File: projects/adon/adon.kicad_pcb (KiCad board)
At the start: 2 copper layers, 55.9 x 30.5 mm, 31 parts, among them IC1 STM32F030F4, P1 BATTERY, P2 SWD, Q1 2N3704, SW1 POWER, SW2 BUTTON0, SW3 BUTTON1, SW4 BUTTON2, SW5 BUTTON3

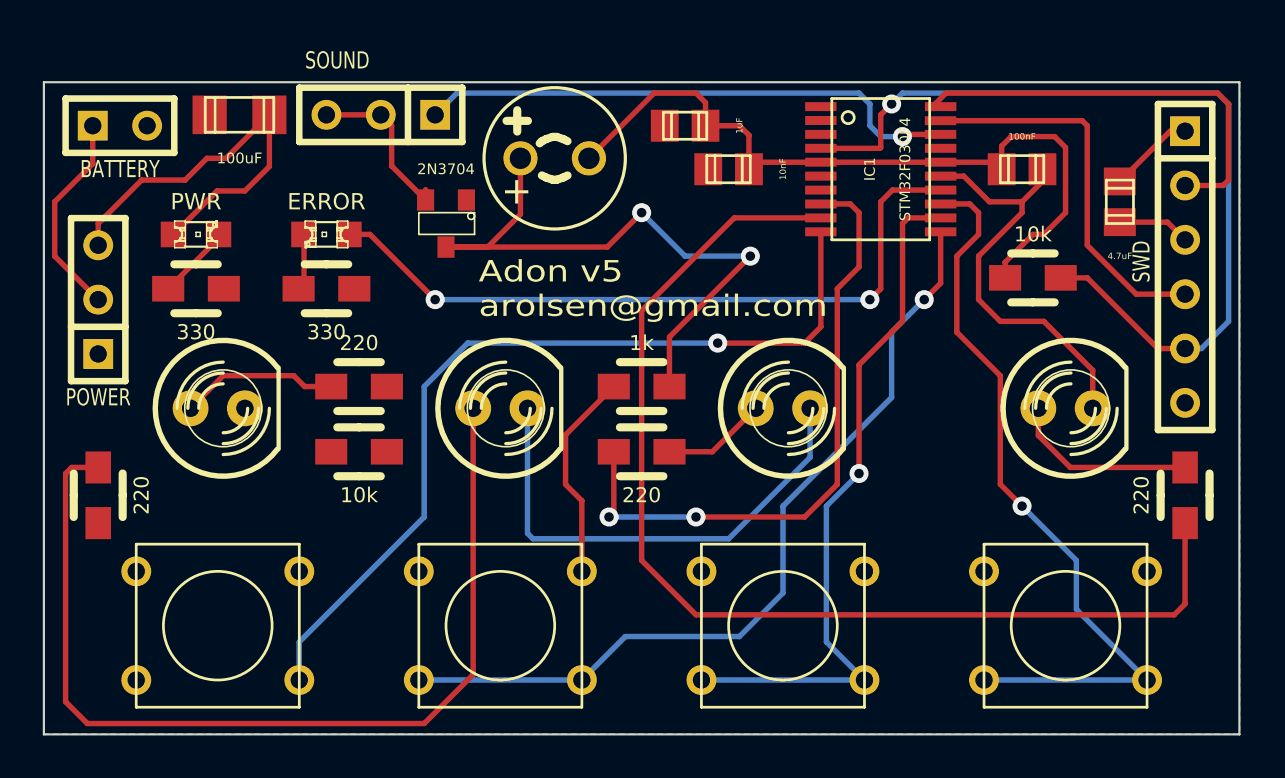
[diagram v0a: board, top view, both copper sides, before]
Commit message: done
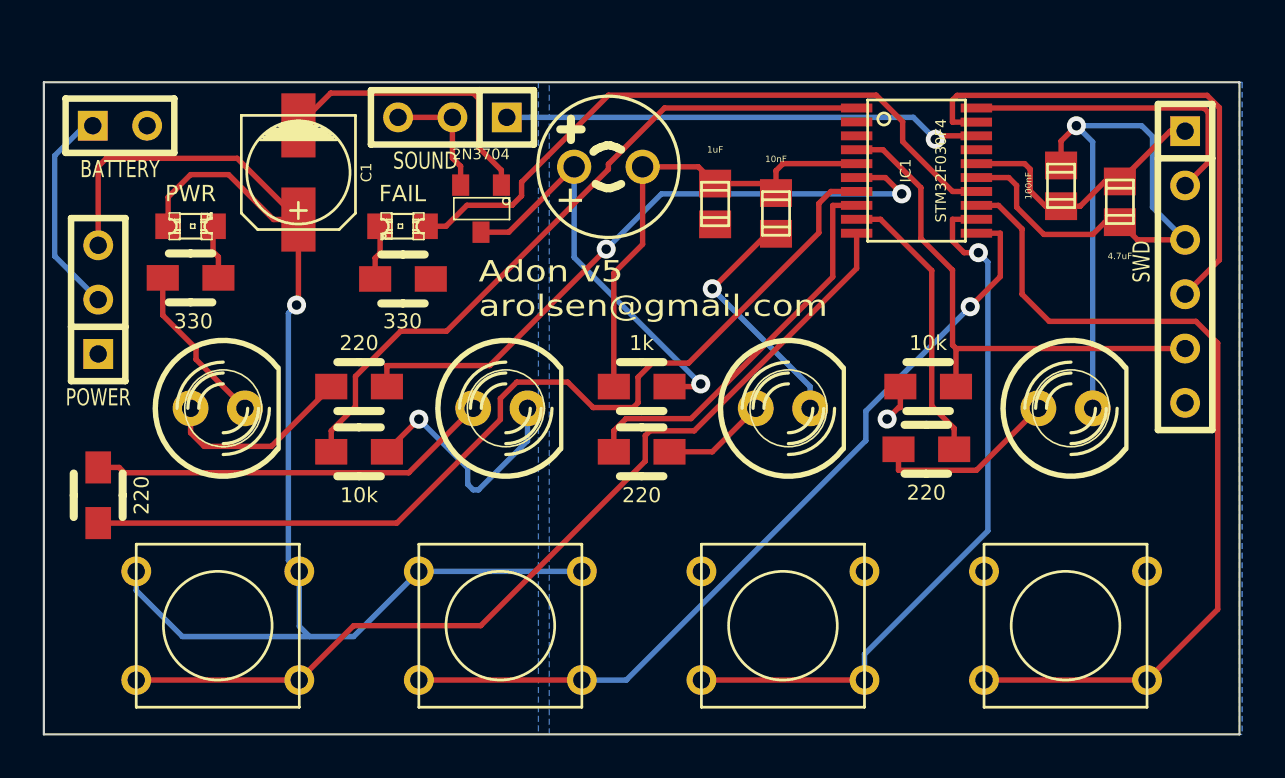
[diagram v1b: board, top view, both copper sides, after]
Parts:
- C1: footprint Capacitors_SMD:c_1206 -> Capacitors_SMD:c_elec_5x5.3
- D1: value ERROR -> FAIL
- moved R3 12.3 mm to (54.5, 30.4), turned to 180 degrees
- moved R2 7.06 mm to (54.5, 27.4)
- moved C2 3.92 mm to (44.6, 18.9), turned to 90 degrees
- moved C1 3.85 mm to (25.1, 17.4), turned to 270 degrees
- moved R9 3.61 mm to (30.0, 22.4)
- moved D1 3.58 mm to (30.0, 19.9)
- moved JP1 3.35 mm to (32.3, 14.8)
- moved C4 3.03 mm to (47.4, 19.3), turned to 270 degrees
- moved SP1 2.54 mm to (39.6, 17.2)
- moved C5 1.98 mm to (60.8, 18.0), turned to 90 degrees
- moved Q1 1.78 mm to (33.6, 19.1)
- moved IC1 1.67 mm to (54.0, 17.3)
- moved R8 0.57 mm to (20.1, 22.4), turned to 180 degrees
- moved D6 0.46 mm to (20.1, 19.9)
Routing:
- net Net-(IC1-Pad7): track 0.00 -> 44.9 mm
- net Net-(IC1-Pad9): track 52.3 -> 13.3 mm
- net VDD: track 69.1 -> 104.1 mm, vias 0 -> 2
- net GND: track 46.5 -> 81.3 mm, vias 0 -> 3
- net Net-(IC1-Pad1): track 0.00 -> 32.8 mm
- net Net-(IC1-Pad6): track 0.00 -> 30.8 mm, vias 0 -> 2
- net Net-(D4-Pad1): track 45.9 -> 18.9 mm
- net NRST: track 41.1 -> 24.4 mm, vias 1 -> 0
- net Net-(IC1-Pad8): track 29.5 -> 18.7 mm, vias 2 -> 0
- net Net-(Q1-Pad3): track 30.1 -> 19.7 mm, vias 2 -> 1
- net SWDIO: track 18.1 -> 24.3 mm
- net SWCLK: track 20.2 -> 14.8 mm
- net Net-(IC1-Pad13): track 35.5 -> 40.5 mm, vias 1 -> 0
- net Net-(IC1-Pad10): track 40.3 -> 44.0 mm, vias 1 -> 0
- net Net-(IC1-Pad18): track 25.5 -> 22.4 mm
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- added copper zone on B.Cu, net GND
